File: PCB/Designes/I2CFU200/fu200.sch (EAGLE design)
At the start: 26 parts, among them IC2 LM358N, K1 FINDER-30.22, K2 FINDER-30.22, K3 FINDER-30.22, Q1 BS170, Q2 BS170, Q3 BS170, U1 ATMEGA328P-AU, X1 250-111, X2 250-111, X3 250-102

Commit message: FU200
Freuquenzumrichter als neues Device erstellt, Transistoren und wagt
klemmen hinzugefügt
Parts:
- removed D1, D2, D3: 1N4148DO35-10, diode:1N4148DO35-10
- removed K1, K2, K3: FINDER-30.22, relay:FINDER-30.22
- removed Q1, Q2, Q3: BS170, transistor-small-signal:BS170
- removed R6, R7, R8: 100, SparkFun-Resistors:100KOHM-1/10W-1%(0603)
- removed X2: 250-111, con-wago_250:250-111
- added T1, T2, T3: 2N3565, transistor:2N3565
- added U$2: HUN_FU2, Btz:HUN_FU2
- R1, R2, R3: value 100k -> 4,7k; device SparkFun-Resistors:100KOHM-1/10W-1%(0603) -> resistor:R-EU_0309/10
- X3: value 250-102 -> 250-706; device con-wago_250:250-102 -> con-wago_250:250-706
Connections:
- removed net N$14: K1-1.O, X1.P3
- removed net N$18: K2-1.O, X1.P6
- removed net N$19: K2-1.P, X1.P7
- removed net N$20: K2-1.S, X1.P8
- removed net N$21: K3-1.O, X1.P9
- removed net N$22: K3-1.P, X1.P10
- removed net N$23: K3-1.S, X1.P11
- removed net N$24: K1-2.P, X2.P2
- removed net N$25: K1-2.S, X2.P3
- removed net N$26: K2-2.O, X2.P4
- removed net N$27: K2-2.P, X2.P5
- removed net N$28: K2-2.S, X2.P6
- removed net N$29: K3-2.O, X2.P7
- removed net N$30: K3-2.P, X2.P8
- removed net N$31: K3-2.S, X2.P9
- removed net N$36: Q1.G, R8.2
- removed net N$38: Q2.G, R7.2
- removed net N$40: IC2A.OUT, R4.2, X3.P1
- removed net N$41: Q3.G, R6.2
- new net 0-10V: IC2A.OUT, R4.2, X3.P1.1
- new net DIR: X3.P5.2
- new net EN: X3.P4.2
- new net FOR: T3.C, X3.P5.1
- new net GND: MCP4811.7, R5.1, T1.E, T2.E, T3.E, U$1.GND, U1.GND, U1.GND_2, U1.GND_3, X1.P2, X3.P2.1, X3.P6.1, X3.P6.2
- new net PUL: X3.P3.2
- new net RES: T1.C, X3.P3.1
- new net REV: T2.C, X3.P4.1
- net N$1: now also U1.PB0_D8; no longer D1.A, K1K.2, Q1.D
- net N$11: now also U$2.REV(INPUT); no longer K1-2.O, X2.P1
- net N$12: no longer R7.1
- net N$13: now also JP1.2, MCP4811.1, MCP4811.6, U1.VCC, U1.VCC_2, X1.P1; no longer MCP4811.7, Q1.S, Q2.S, Q3.S, R1.2, R2.2, R3.2, R5.1, U$1.GND, U1.GND, U1.GND_2, U1.GND_3, X3.P2
- net N$15: no longer R6.1
- net N$16: now also R2.2, T2.B; no longer K1-1.P, X1.P4
- net N$17: now also U$2.ACM(0V/GND)?; no longer K1-1.S, X1.P5
- net N$2: now also R1.2, T1.B; no longer JP1.2, MCP4811.1, MCP4811.6, U1.VCC_2
- net N$3: now also U$2.DCM(0V/GND)?; no longer R1.1, R8.1
- net N$5: now also R3.2, T3.B; no longer D1.C, D2.C, D3.C, K1K.1, K2K.1, K3K.1
- net N$8: now also U$2.RST; no longer D2.A, K2K.2, Q2.D
- net N$9: now also U$2.FOR(INPUT); no longer D3.A, K3K.2, Q3.D
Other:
- note added: "+5V Externe Spannungsversorgung (Optional)"
- note removed: "+ 5V"
- note removed: "-"
- moved on the sheet: IC2A, MCP4811, R4, R5, U$1, X1

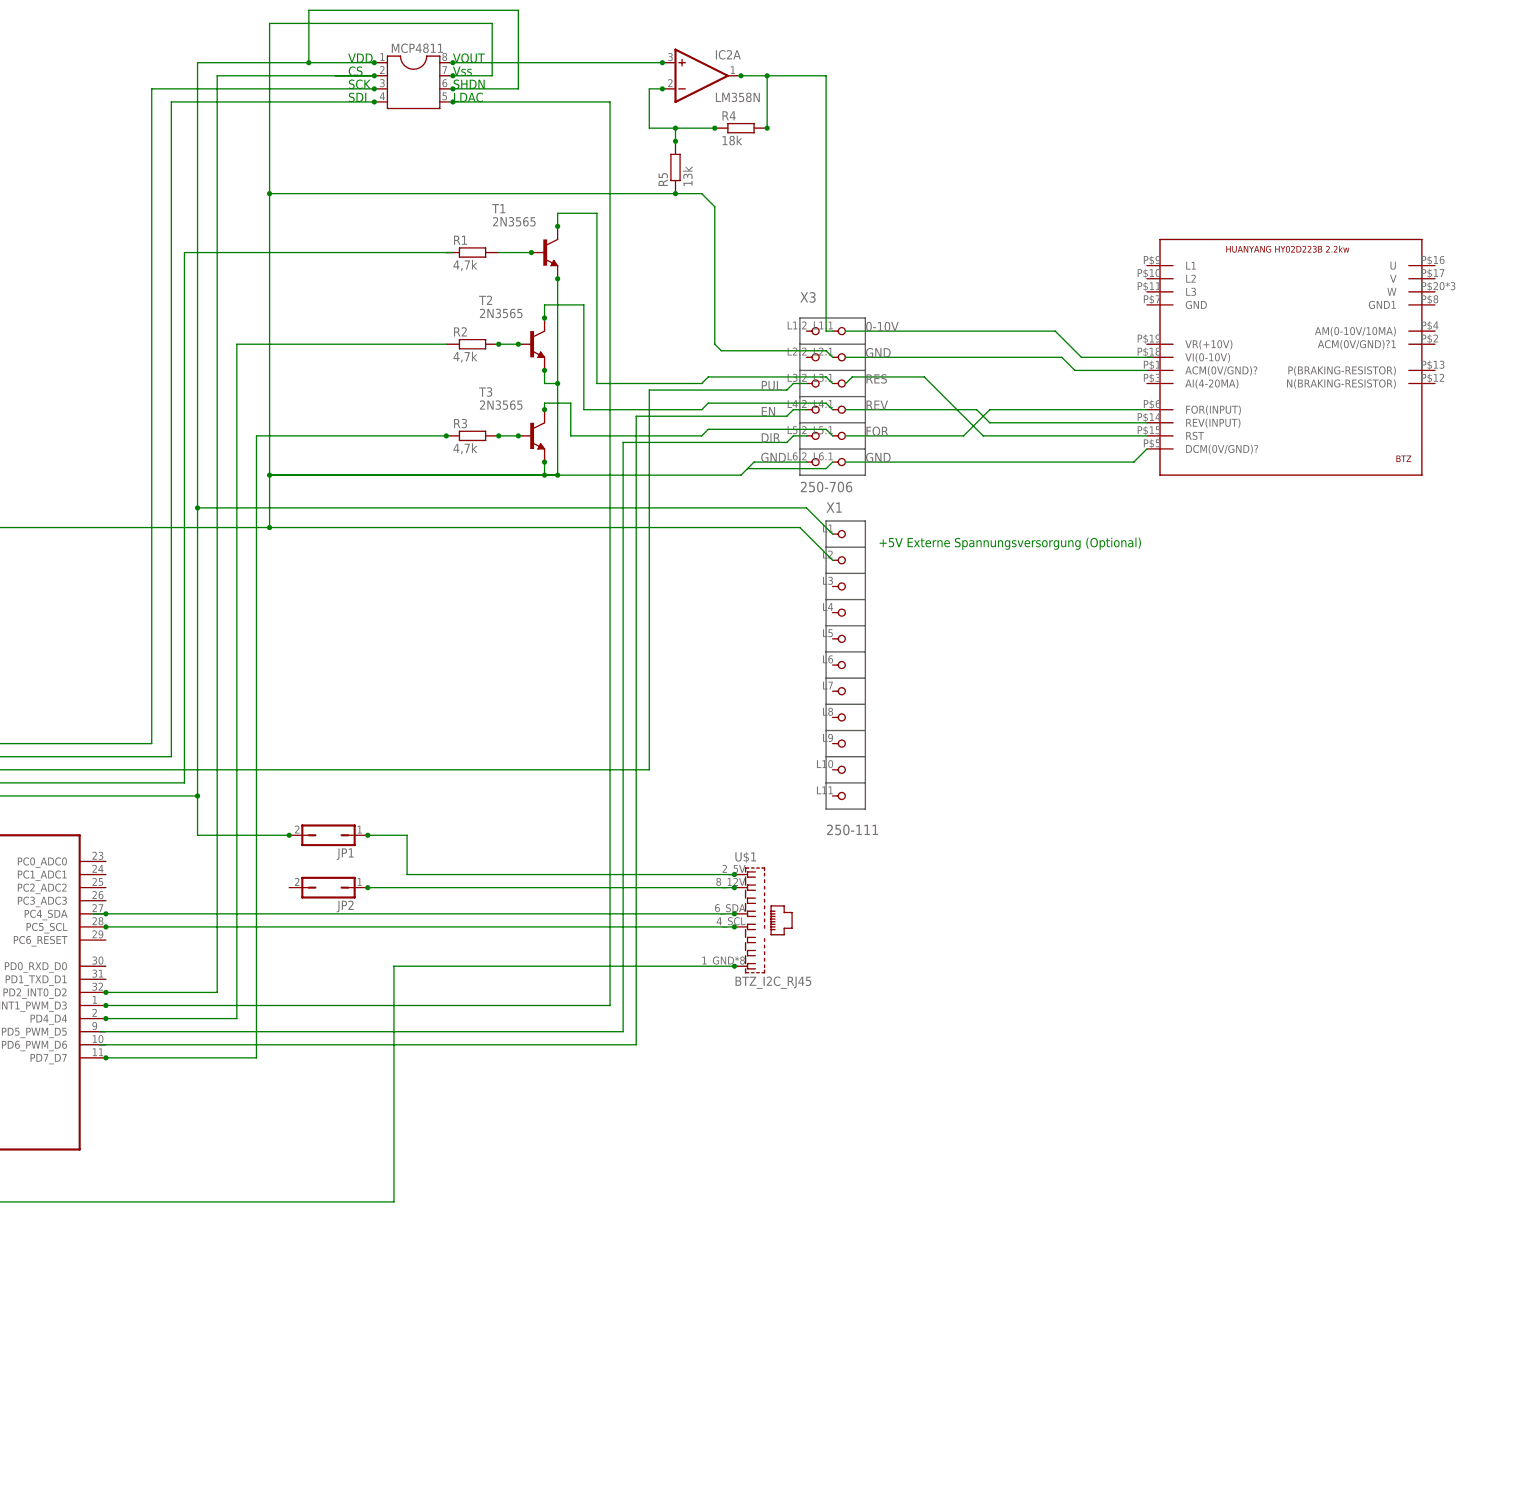
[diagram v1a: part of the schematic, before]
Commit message: ++
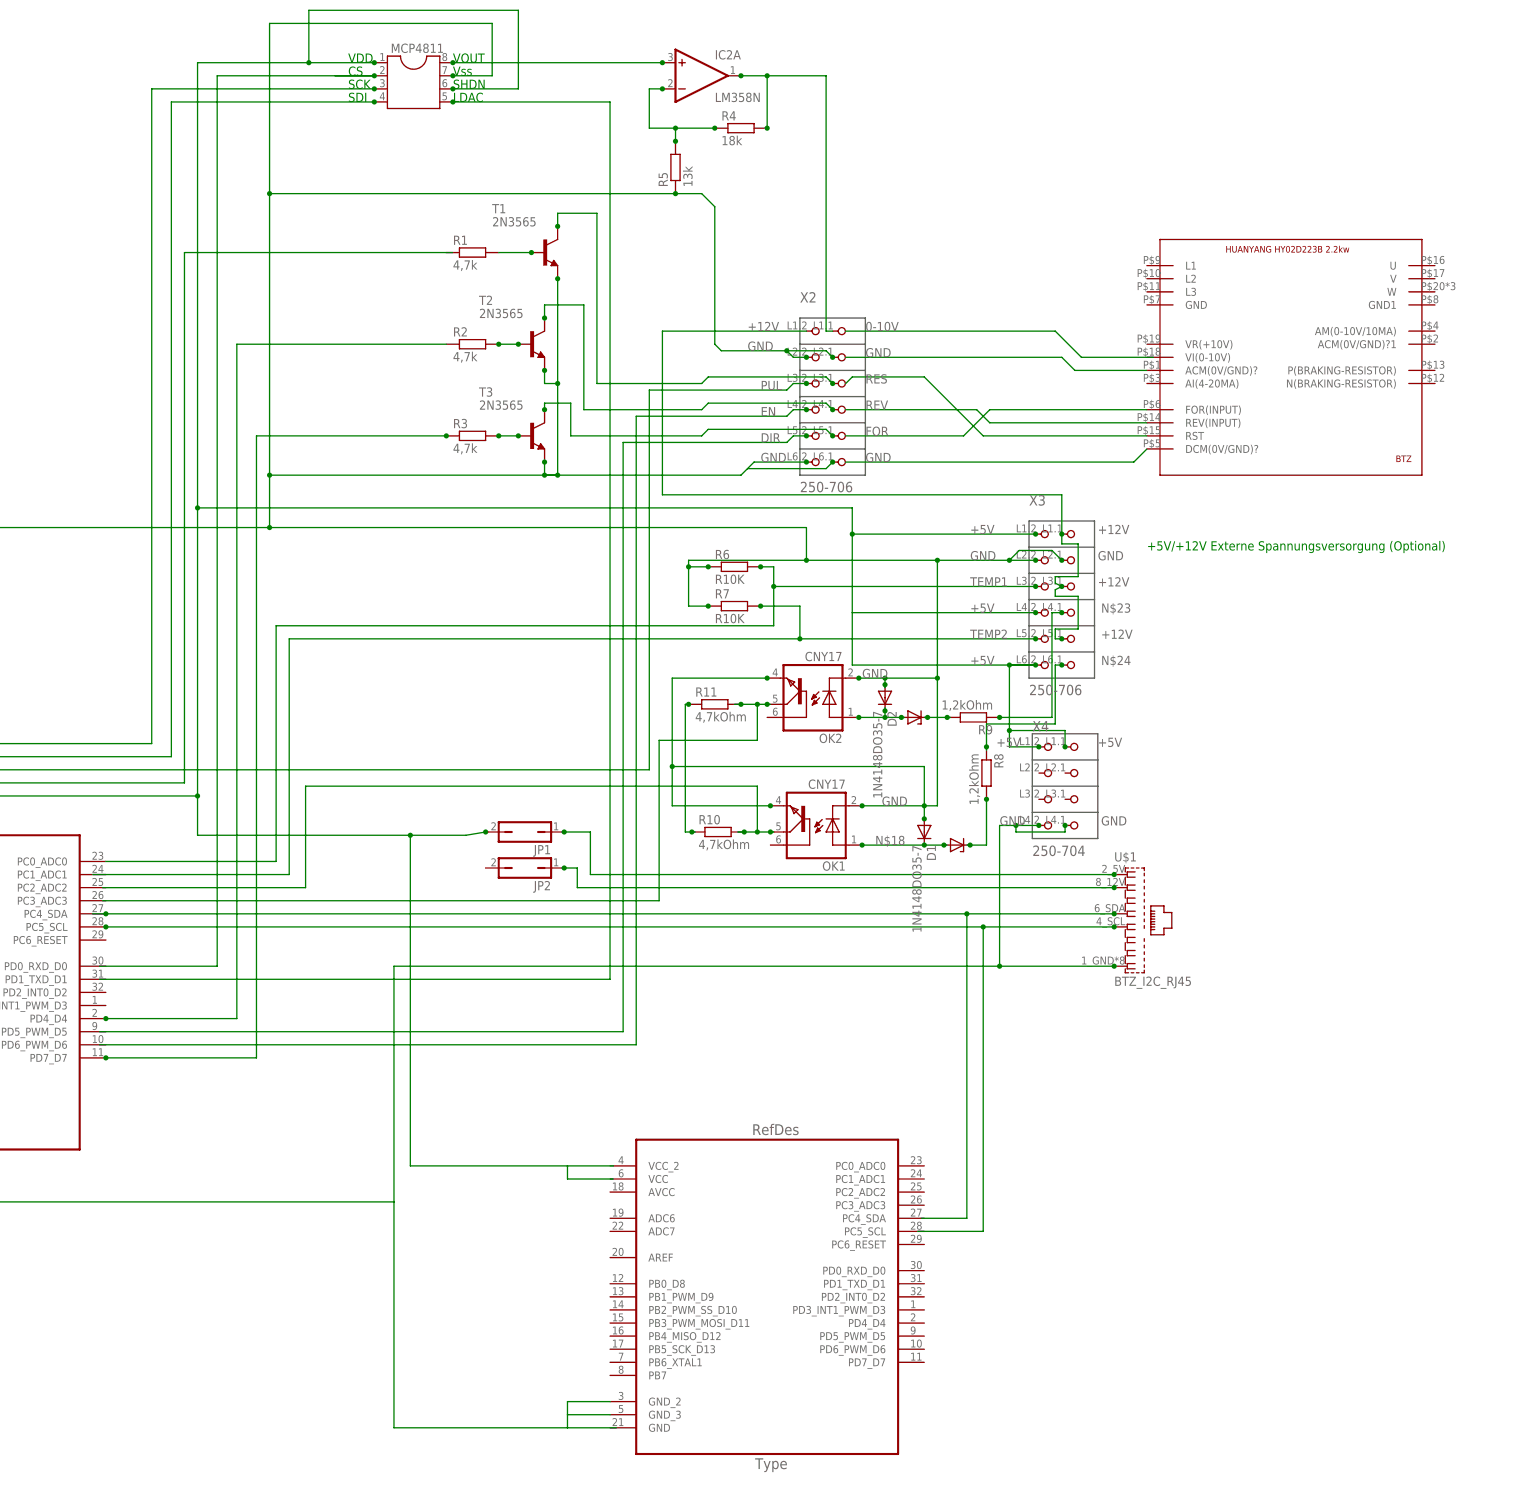
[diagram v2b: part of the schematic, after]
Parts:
- removed X1: 250-111, con-wago_250:250-111
- added D1, D2: 1N4148DO35-7, diode:1N4148DO35-7
- added OK1, OK2: CNY17, optocoupler:CNY17
- added R10, R11: 4,7kOhm, resistor:R-EU_0204/7
- added R6, R7: R10K, resistor:R-EU_0309/10
- added R8, R9: 1,2kOhm, resistor:R-EU_0204/7
- added U2: ATMEGA328P-AU, Atmel-ATMEGA328P-AU:ATMEGA328P-AU
- added X2: 250-706, con-wago_250:250-706
- added X4: 250-704, con-wago_250:250-704
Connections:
- new net +12V: X2.P1.2, X3.P1.1, X3.P3.1, X3.P5.1
- new net +5V: JP1.2, MCP4811.1, MCP4811.6, U1.VCC, U1.VCC_2, X3.P1.2, X3.P4.2, X3.P6.2, X4.P1.1, X4.P1.2
- new net N$18: D1.C, OK1.A
- new net N$19: D2.C, OK2.A
- new net N$20: R9.2
- new net N$21: R10.1, R11.1
- new net N$22: OK2.COL, R11.2
- new net N$23: R9.1, X3.P4.1
- new net N$24: R8.1, X3.P6.1
- new net N$25: OK1.COL, R10.2
- new net TEMP1: R6.2, U1.PC0_ADC0, X3.P3.2
- new net TEMP2: R7.2, X3.P5.2
- net 0-10V: now also X2.P1.1; no longer X3.P1.1
- net DIR: now also X2.P5.2; no longer X3.P5.2
- net EN: now also X2.P4.2; no longer X3.P4.2
- net FOR: now also X2.P5.1; no longer X3.P5.1
- net GND: now also D1.A, D2.A, OK1.C, OK1.EMI, OK2.C, OK2.EMI, R6.1, R7.1, U2.GND_2, U2.GND_3, X2.P2.1, X2.P2.2, X2.P6.1, X2.P6.2, X3.P2.2, X4.P4.1, X4.P4.2; no longer X1.P2, X3.P6.1, X3.P6.2
- net N$13: now also R8.2; no longer JP1.2, MCP4811.1, MCP4811.6, U1.VCC, U1.VCC_2, X1.P1
- net N$32: no longer U1.PD2_INT0_D2
- net N$37: no longer U1.PD3_INT1_PWM_D3
- net PUL: now also X2.P3.2; no longer X3.P3.2
- net RES: now also X2.P3.1; no longer X3.P3.1
- net REV: now also X2.P4.1; no longer X3.P4.1
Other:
- note added: "+5V/+12V Externe Spannungsversorgung (Optional)"
- note removed: "+5V Externe Spannungsversorgung (Optional)"
- moved on the sheet: JP1, JP2, U$1, X3
